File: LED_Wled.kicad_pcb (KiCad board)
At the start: 2 copper layers, 100 x 97.5 mm, 131 parts, among them J1 SWD_PORT_SKEDD, J2 Screw_Terminal_01x02, J3 Screw_Terminal_01x03, Q1 BSS138, U1 ESP8266-12E_ESP-12E, U2 AMS1117-3.3, U3 AMS1117-5.0

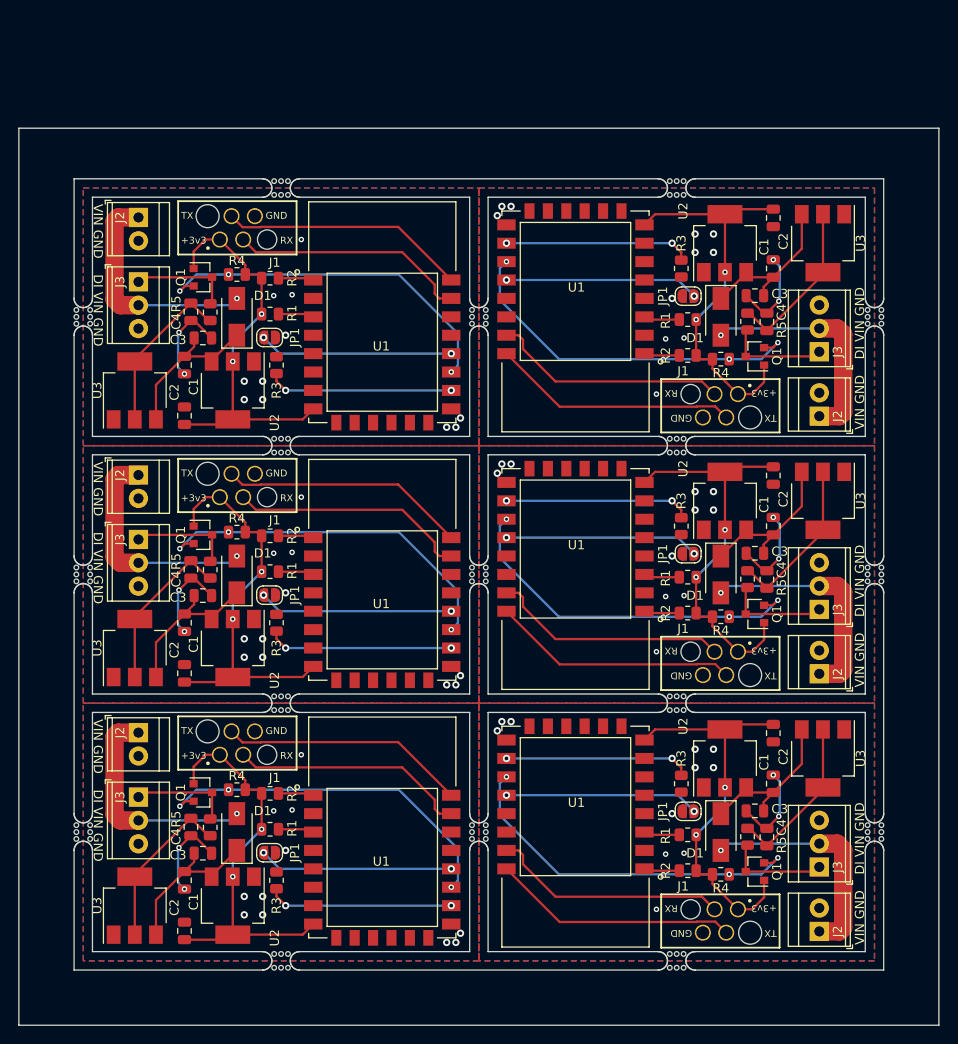
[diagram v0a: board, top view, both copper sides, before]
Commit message: updated to rev1.1
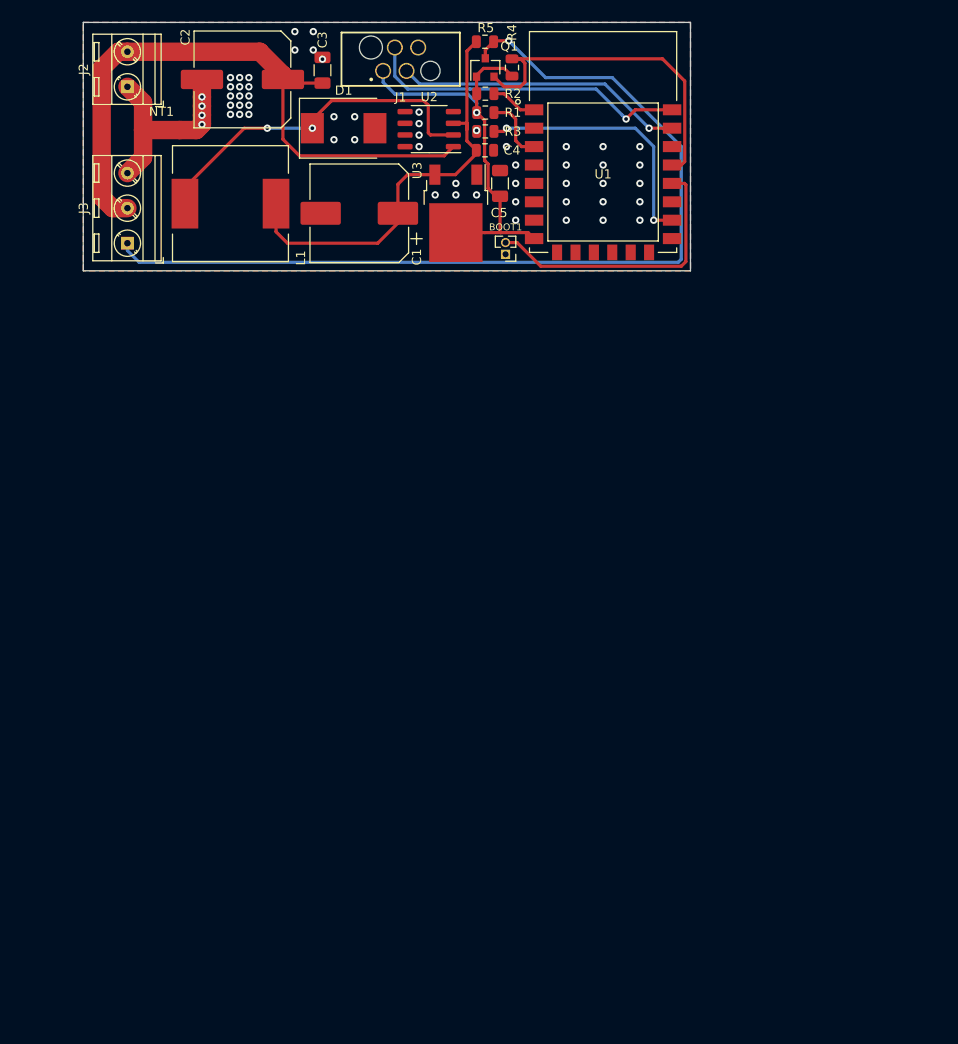
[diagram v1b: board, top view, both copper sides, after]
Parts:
- removed the C1 at (142.0, 128.8)
- removed the C1 at (78.0, 139.2)
- removed the C1 at (142.0, 100.8)
- removed the C1 at (78.0, 111.2)
- removed the C1 at (142.0, 72.8)
- removed the C1 at (78.0, 83.2)
- removed the C2 at (142.0, 123.2)
- removed the C2 at (78.0, 144.8)
- removed the C2 at (142.0, 95.2)
- removed the C2 at (78.0, 116.8)
- removed the C2 at (142.0, 67.2)
- removed the C2 at (78.0, 88.8)
- removed the C3 at (140.0, 131.7)
- removed the C3 at (80.0, 136.3)
- removed the C3 at (140.0, 103.7)
- removed the C3 at (80.0, 108.3)
- removed the C3 at (140.0, 75.7)
- removed the C3 at (80.0, 80.3)
- removed the C4 at (141.3, 134.6)
- removed the C4 at (78.7, 133.4)
- removed the C4 at (141.3, 106.5)
- removed the C4 at (78.7, 105.5)
- removed the C4 at (141.3, 78.5)
- removed the C4 at (78.7, 77.5)
- removed the D1 at (136.3, 134.0)
- removed the D1 at (83.7, 134.0)
- removed the D1 at (136.3, 106.0)
- removed the D1 at (83.7, 106.0)
- removed the D1 at (136.3, 78.0)
- removed the D1 at (83.7, 78.0)
- removed G*** (x6): LOGO, LED_Wled:es
- removed the J1 at (136.2, 143.7)
- removed the J1 at (83.8, 124.3)
- removed the J1 at (136.2, 115.7)
- removed the J1 at (83.8, 96.3)
- removed the J1 at (136.2, 87.7)
- removed the J1 at (83.8, 68.3)
- removed the J2 at (147.0, 144.8)
- removed the J2 at (73.0, 123.2)
- removed the J2 at (147.0, 116.8)
- removed the J2 at (73.0, 95.2)
- removed the J2 at (147.0, 88.8)
- removed the J2 at (73.0, 67.2)
- removed the J3 at (147.0, 137.8)
- removed the J3 at (73.0, 130.2)
- removed the J3 at (147.0, 109.8)
- removed the J3 at (73.0, 102.2)
- removed the J3 at (147.0, 81.8)
- removed the J3 at (73.0, 74.2)
- removed JP1 (x6): Jumper, Jumper:SolderJumper-2_P1.3mm_Open_RoundedPad1.0x1.5mm
- removed the Q1 at (140.0, 138.3)
- removed the Q1 at (80.0, 129.7)
- removed the Q1 at (140.0, 110.3)
- removed the Q1 at (80.0, 101.7)
- removed the Q1 at (140.0, 82.3)
- removed the Q1 at (80.0, 73.7)
- removed the R1 at (132.7, 134.3)
- removed the R1 at (87.3, 133.7)
- removed the R1 at (132.7, 106.3)
- removed the R1 at (87.3, 105.7)
- removed the R1 at (132.7, 78.3)
- removed the R1 at (87.3, 77.7)
- removed the R2 at (132.7, 138.2)
- removed the R2 at (87.3, 129.8)
- removed the R2 at (132.7, 110.2)
- removed the R2 at (87.3, 101.8)
- removed the R2 at (132.7, 82.2)
- removed the R2 at (87.3, 73.8)
- removed the R3 at (132.0, 128.8)
- removed the R3 at (88.0, 139.2)
- removed the R3 at (132.0, 100.8)
- removed the R3 at (88.0, 111.2)
- removed the R3 at (132.0, 72.8)
- removed the R3 at (88.0, 83.2)
- removed the R4 at (136.3, 138.6)
- removed the R4 at (83.7, 129.4)
- removed the R4 at (136.3, 110.6)
- removed the R4 at (83.7, 101.4)
- removed the R4 at (136.3, 82.6)
- removed the R4 at (83.7, 73.4)
- removed the R5 at (139.2, 134.5)
- removed the R5 at (80.8, 133.5)
- removed the R5 at (139.2, 106.5)
- removed the R5 at (80.8, 105.5)
- removed the R5 at (139.2, 78.5)
- removed the R5 at (80.8, 77.5)
- removed the U1 at (120.5, 131.0)
- removed the U1 at (99.5, 137.0)
- removed the U1 at (120.5, 103.0)
- removed the U1 at (99.5, 109.0)
- removed the U1 at (120.5, 75.0)
- removed the U1 at (99.5, 81.0)
- removed the U2 at (136.8, 126.0)
- removed the U2 at (83.2, 142.0)
- removed the U2 at (136.8, 98.0)
- removed the U2 at (83.2, 114.0)
- removed the U2 at (136.8, 70.0)
- removed the U2 at (83.2, 86.0)
- removed the U3 at (147.4, 126.0)
- removed the U3 at (72.6, 142.0)
- removed the U3 at (147.4, 98.0)
- removed the U3 at (72.6, 114.0)
- removed the U3 at (147.4, 70.0)
- removed the U3 at (72.6, 86.0)
- removed mouse-bite-2mm-slot (x17): VAL**, Panelization:mouse-bite-2mm-slot
- added BOOT1: Jumper, Connector_PinHeader_1.27mm:PinHeader_1x02_P1.27mm_Vertical, F.Cu at (112.9, 71.2)
- added C1: 180uF/35V, Capacitor_SMD:CP_Elec_10x12.5, F.Cu at (97.0, 66.8)
- added C2: 470uF/35V, Capacitor_SMD:C_Elec_10x10.2, F.Cu at (84.3, 52.2)
- added C3: 1uF/50V, Capacitor_SMD:C_1206_3216Metric, F.Cu at (93.0, 51.2)
- added C4: 100nF/50V, Capacitor_SMD:C_0805_2012Metric, F.Cu at (110.7, 59.9)
- added C5: 10uF/50V, Capacitor_SMD:C_1206_3216Metric, F.Cu at (112.3, 63.5)
- added D1: SS32, Diode_SMD:D_SMC, F.Cu at (95.3, 57.5)
- added J1: SWD_PORT_SKEDD, LED_Wled:WR_WST_REDFIT_IDC_4Pin, F.Cu at (101.5, 50.0)
- added J2: Screw_Terminal_01x02, TerminalBlock_MetzConnect:TerminalBlock_MetzConnect_Type086_RT03402HBLC_1x02_P3.81mm_Horizontal, F.Cu at (71.8, 53.0)
- added J3: Screw_Terminal_01x03, TerminalBlock_MetzConnect:TerminalBlock_MetzConnect_Type086_RT03403HBLC_1x03_P3.81mm_Horizontal, F.Cu at (71.8, 70.0)
- added L1: 68uH, Inductor_SMD:L_12x12mm_H8mm, F.Cu at (83.0, 65.7)
- added NT1: Net-Tie_2, NetTie:NetTie-2_SMD_Pad2.0mm, F.Cu at (75.5, 57.7)
- added Q1: BSS138, Package_TO_SOT_SMD:SOT-23, F.Cu at (110.7, 50.9)
- added R1: 10k, Resistor_SMD:R_0805_2012Metric, F.Cu at (110.7, 55.8)
- added R2: 10k, Resistor_SMD:R_0805_2012Metric, F.Cu at (110.7, 53.8)
- added R3: 10k, Resistor_SMD:R_0805_2012Metric, F.Cu at (110.7, 57.9)
- added R4: 10k, Resistor_SMD:R_0805_2012Metric, F.Cu at (113.6, 50.9)
- added R5: 10k, Resistor_SMD:R_0805_2012Metric, F.Cu at (110.7, 48.1)
- added U1: ESP8266-12E_ESP-12E, LED_Wled:ESP-12E, F.Cu at (123.5, 62.5)
- added U2: XL1509, Package_SO:SOP-8_3.9x4.9mm_P1.27mm, F.Cu at (104.6, 57.6)
- added U3: LD1117DT33TR, Package_TO_SOT_SMD:TO-252-2, F.Cu at (107.5, 66.8)
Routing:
- net (no net): track 1340.2 -> 0.00 mm, vias 115 -> 0
- net LED_OUT_HV: track 11.2 -> 101.3 mm, vias 0 -> 1
- net VIN: track 25.1 -> 69.9 mm, vias 1 -> 0
- net Net-(D1-Pad1): track 0.00 -> 38.7 mm, vias 0 -> 2
- net Net-(BOOT1-Pad2): track 0.00 -> 30.8 mm
- net +5V: track 18.1 -> 47.0 mm
- net Net-(JP1-Pad2): track 21.1 -> 0.00 mm, vias 2 -> 0
- net /PROT_VIN: track 18.5 -> 0.00 mm
- net GNDPWR: track 0.00 -> 10.8 mm
- net TXD: track 26.8 -> 35.6 mm, vias 0 -> 1
- net Net-(R3-Pad1): track 20.3 -> 28.3 mm
- net RXD: track 25.9 -> 31.4 mm, vias 0 -> 1
- net Net-(R1-Pad2): track 3.91 -> 7.27 mm
- net LED_OUT_LV: track 39.8 -> 37.7 mm, vias 3 -> 0
- net GND: track 9.71 -> 7.65 mm, vias 13 -> 57
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- removed copper zone on B.Cu, net (none)
- removed copper zone on F.Cu, net (none)
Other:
- board size 100 x 97.5 mm -> 66 x 27 mm
- board text added: "For use with ARGB LED-strip MAX INPUT: +30 V"
- board text added: "remote-led-project 2022-01-13 rev1.1"
- board text removed: "+3v3"
- board text removed: "DI VIN GND"
- board text removed: "For use with ARGB LED-strip MAX INPUT: +13V"
- board text removed: "GND"
- board text removed: "RX"
- board text removed: "TX"
- board text removed: "VIN GND"
- board text removed: "remote-led-project 2021-11-04 rev1.0"
